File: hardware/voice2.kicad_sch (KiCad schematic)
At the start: 30 parts, among them IC1 LM13700, U12 MCP4922-E/P, U13 SSM2044

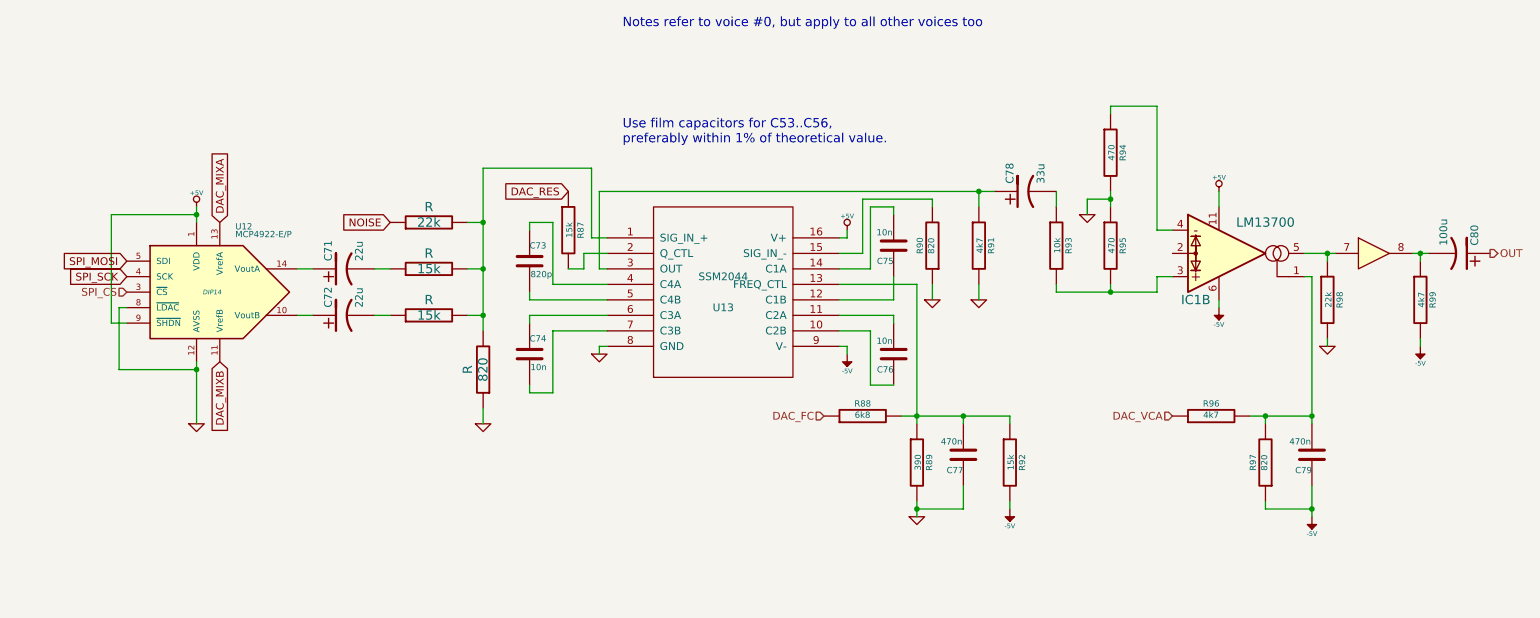
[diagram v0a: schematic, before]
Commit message: hardware: SSM2044 -> SSI2144
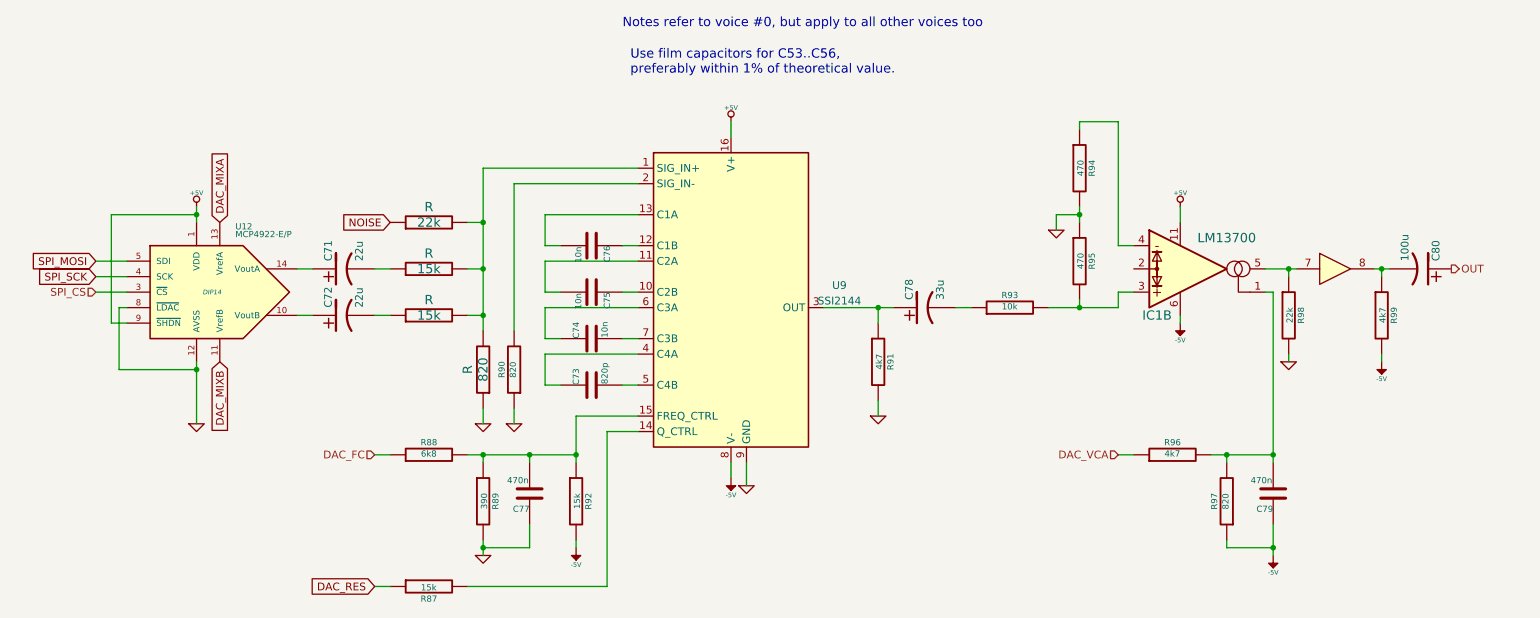
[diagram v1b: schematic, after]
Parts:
- removed U13: SSM2044, MODULE, symbol overcycler2-rescue:SSM2044
- added U9: SSI2144, Package_SO:SSOP-16_3.9x4.9mm_P0.635mm, symbol Audio:SSI2144
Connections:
- net +5V: now also U9.16 (V+)
- net -5V: now also U9.8 (V-)
- net GND: now also U9.9 (GND)
- net at R.2, R.2, R.2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: now also U9.1 (SIG_IN+)
- net at C76.1: now also U9.12 (C1B)
- net at C76.2: now also U9.13 (C1A)
- net at C75.1: now also U9.10 (C2B)
- net at C77.2, R88.2, R89.1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: now also U9.15 (FREQ_CTRL)
- net at C75.2: now also U9.11 (C2A)
- net at R90.2: now also U9.2 (SIG_IN-)
- net at R87.2: now also U9.14 (Q_CTRL)
- net at C78.1, R91.1: now also U9.3 (OUT)
- net at C73.1: now also U9.4 (C4A)
- net at C73.2: now also U9.5 (C4B)
- net at C74.1: now also U9.6 (C3A)
- net at C74.2: now also U9.7 (C3B)
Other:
- moved on the sheet: C73, C74, C75, C76, C77, C78, C79, C80, IC1B, R87, R88, R89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
